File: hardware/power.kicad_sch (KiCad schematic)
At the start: 33 parts, among them J14 Conn_01x02, Q11 DMP3013SFV, Q13 AO3400A, U5 TPS565208, U7 TPS82130SILR

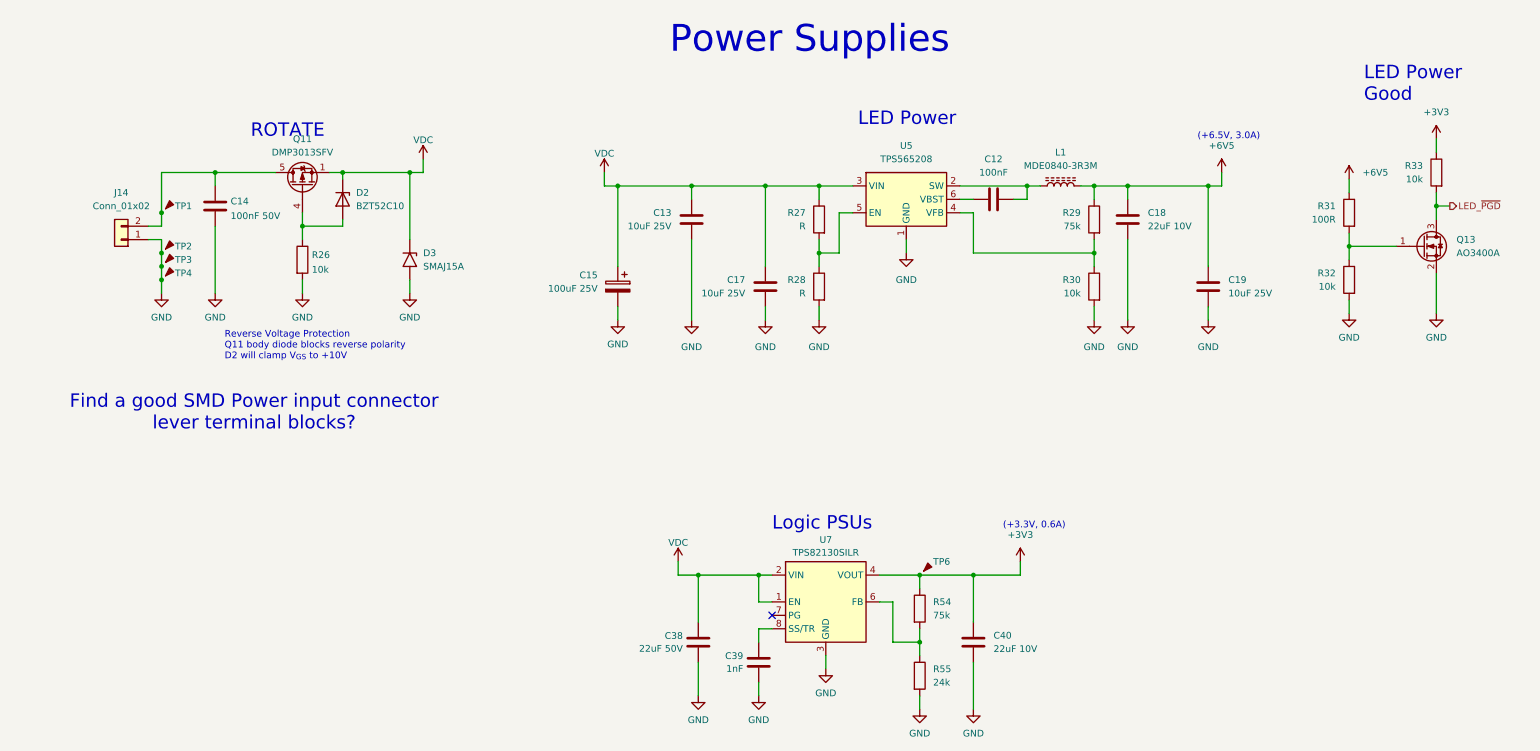
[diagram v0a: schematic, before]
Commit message: some jlc cleanup
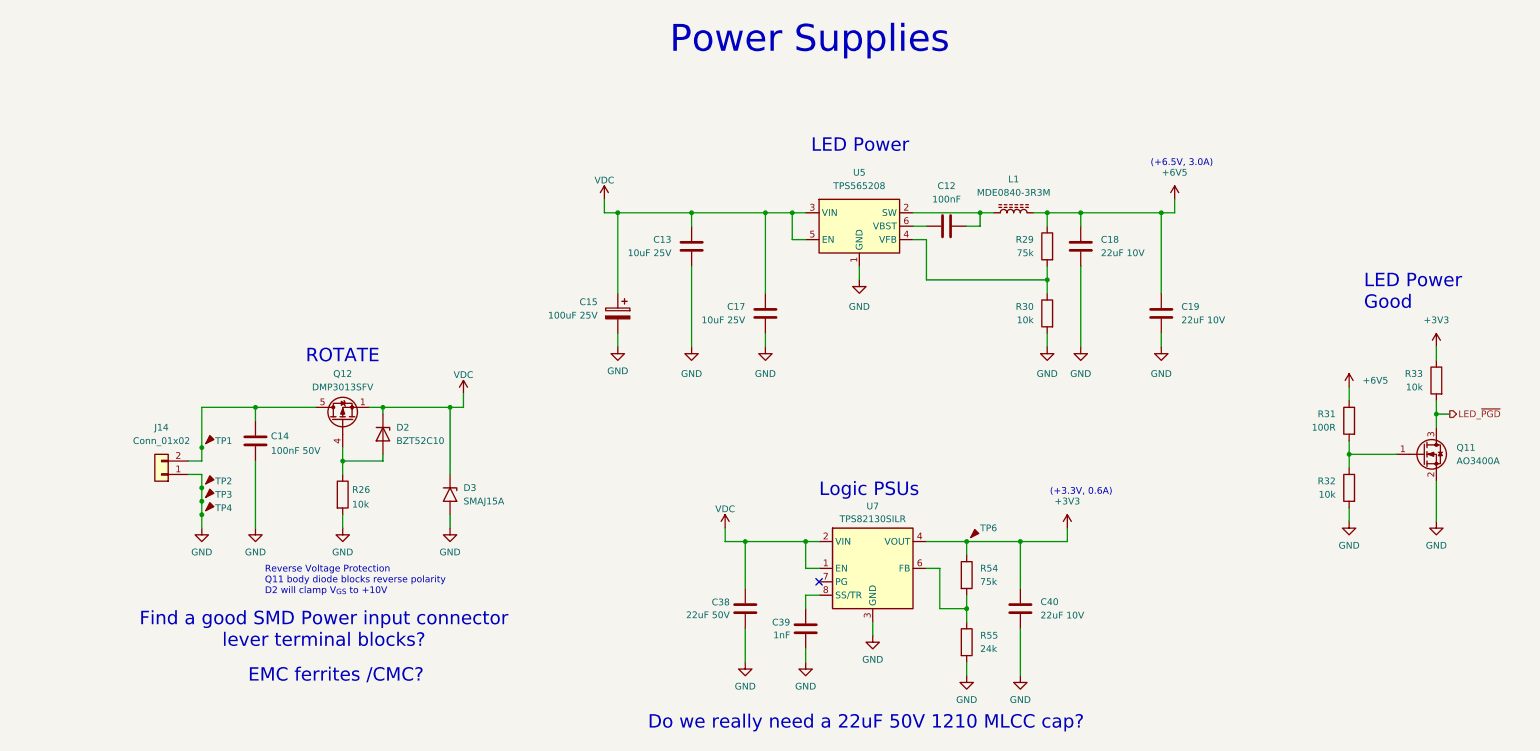
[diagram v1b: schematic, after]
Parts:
- removed R27, R28: R, Resistor_SMD:R_0603_1608Metric, symbol Device:R
- C12: LCSC (none) -> C14663
- C13, C17: LCSC (none) -> C15850
- C15: footprint (none) -> Capacitor_SMD:CP_Elec_6.3x7.7; LCSC (none) -> C72477
- C18: LCSC (none) -> C45783
- C19: value 10uF 25V -> 22uF 10V; LCSC (none) -> C45783
- C39: footprint Capacitor_SMD:C_0402_1005Metric -> Capacitor_SMD:C_0603_1608Metric; LCSC C1523 -> C1588
- C40: LCSC C96123 -> C45783
- J14: footprint Connector_Phoenix_MSTB:PhoenixContact_MSTBVA_2,5_2-G-5,08_1x02_P5.08mm_Vertical -> (none); LCSC (none) -> C7467028
- R26, R30, R32, R33: LCSC C21190 -> C25804
- R29, R54: LCSC (none) -> C23242
- R55: LCSC (none) -> C23352
- renumbered Q13 to Q11, Q11 to Q12
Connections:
- net VDC: now also U5.5 (EN)
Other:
- note added: "Do we really need a 22uF 50V 1210 MLCC cap?"
- note added: "EMC ferrites /CMC?"
- moved on the sheet: C12, C13, C14, C15, C17, C18, C38, C39, C40, D2, D3, J14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
